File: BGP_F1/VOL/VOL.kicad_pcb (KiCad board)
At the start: 2 copper layers, 33 x 30 mm, 26 parts, among them P1 CONN_01X05, P2 CONN_01X05, P3 CONN_01X05, P4 CONN_01X03, P5 CONN_01X02, P7 CONN_01X12, U1 MC33178, U2 MC33178

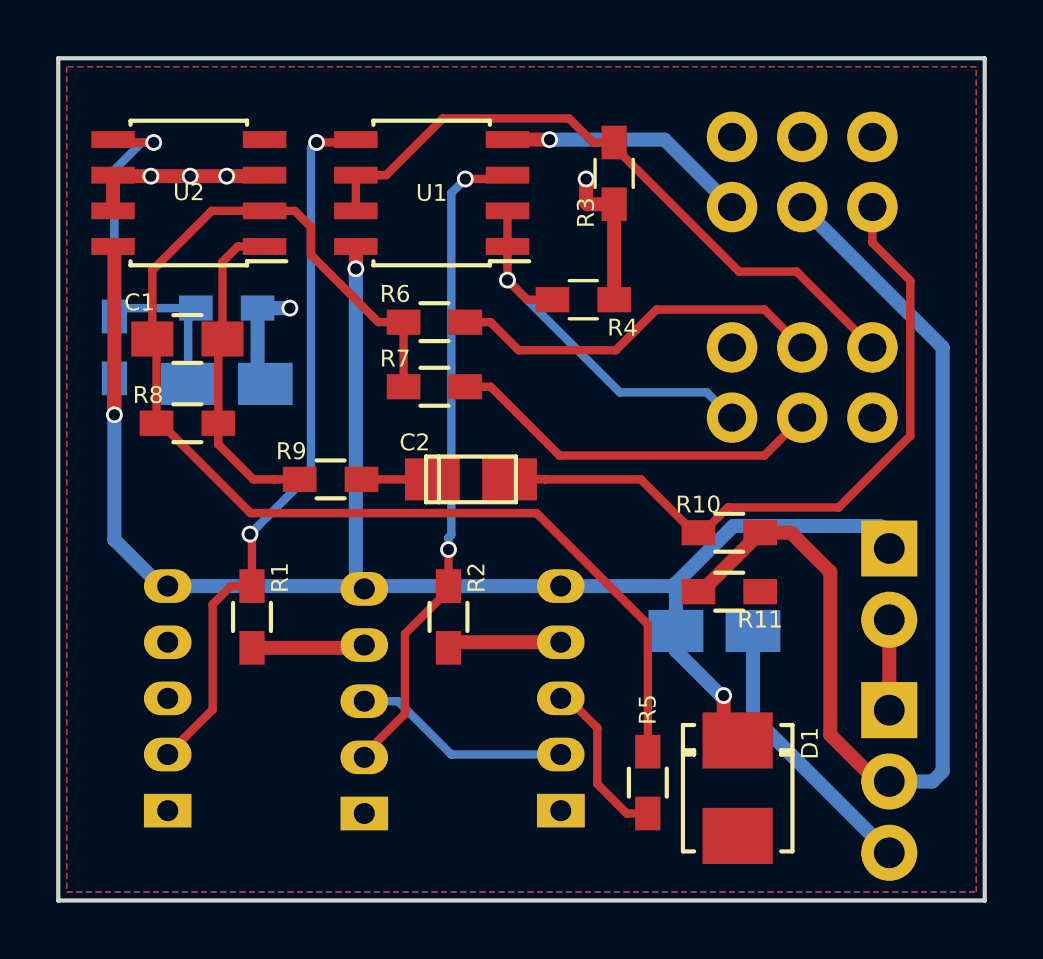
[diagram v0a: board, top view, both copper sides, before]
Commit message: HPF Done
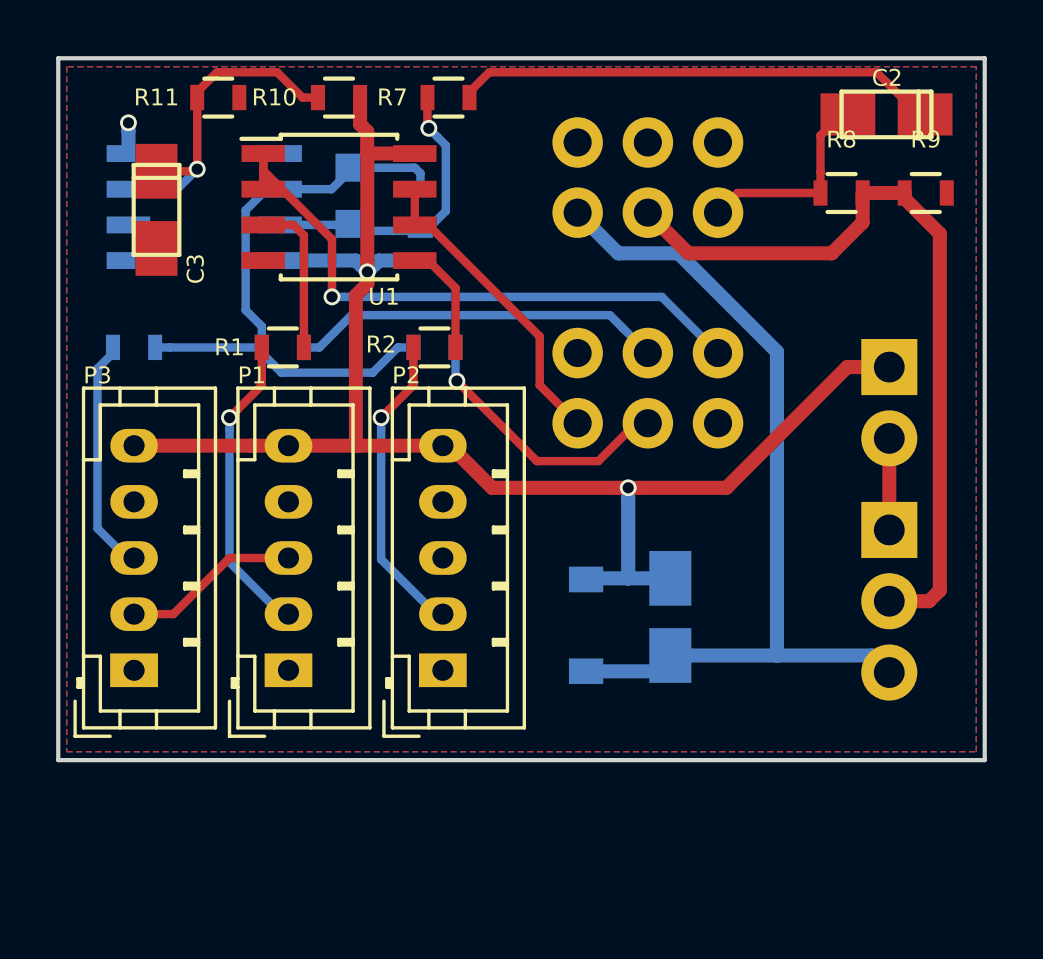
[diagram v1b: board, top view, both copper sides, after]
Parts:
- removed P7: CONN_01X12, LIBS:Potentiometer_Alps_RK097_Quad_Vertical_Dual_Shaft
- removed R12, R13: 100k, Resistors_SMD:R_0603_HandSoldering
- added P6: CONN_01X12, LIBS:Potentiometer_Alps_RK097_Quad_Vertical_Dual_Shaft, B.Cu at (155.5, 79.0)
- C1: footprint Capacitors_SMD:C_0805_HandSoldering -> Capacitors_SMD:C_0805; moved to B.Cu
- C3, P1, P2, P3: moved to F.Cu
- D1: footprint Diodes_SMD:DO-214BA -> Diodes_SMD:SOD-123; moved to B.Cu
- R1, R2: value 249k -> 100; footprint Resistors_SMD:R_0603_HandSoldering -> Resistors_SMD:R_0603
- R10: value 10k -> 100k; footprint Resistors_SMD:R_0603_HandSoldering -> Resistors_SMD:R_0603
- R11: value 12k -> 100k; footprint Resistors_SMD:R_0603_HandSoldering -> Resistors_SMD:R_0603
- R3, R4: value 11.1k -> 47k; footprint Resistors_SMD:R_0603_HandSoldering -> Resistors_SMD:R_0603; moved to B.Cu
- R5, R6: value 4.7k -> 47k; footprint Resistors_SMD:R_0603_HandSoldering -> Resistors_SMD:R_0603; moved to B.Cu
- R7: value 4.7k -> 100; footprint Resistors_SMD:R_0603_HandSoldering -> Resistors_SMD:R_0603
- R8: value 4.7k -> 10k; footprint Resistors_SMD:R_0603_HandSoldering -> Resistors_SMD:R_0603
- R9: value 100 -> 12k; footprint Resistors_SMD:R_0603_HandSoldering -> Resistors_SMD:R_0603
- U2: moved to B.Cu
- moved R11 25.3 mm to (142.7, 77.4)
- moved R8 24.7 mm to (164.9, 80.8), turned to 0 degrees
- moved R9 23.5 mm to (167.9, 80.8), turned to 0 degrees
- moved R10 20.8 mm to (147.0, 77.4), turned to 180 degrees
- moved C2 19.7 mm to (166.5, 78.0), turned to 0 degrees
- moved R3 18.2 mm to (139.7, 86.3), turned to 180 degrees
- moved R5 17.3 mm to (150.4, 86.3), turned to 0 degrees
- moved P3 16.0 mm to (139.7, 97.8)
- moved R4 10.8 mm to (145.0, 86.3), turned to 0 degrees
- moved R7 10.3 mm to (150.9, 77.4), turned to 180 degrees
- moved R1 9.66 mm to (145.0, 86.3), turned to 180 degrees
- moved R2 9.61 mm to (150.4, 86.3), turned to 180 degrees
- moved D1 7.92 mm to (155.8, 96.2)
- moved C1 7.80 mm to (147.5, 80.9), turned to 90 degrees
- moved C3 6.69 mm to (140.5, 81.4), turned to 90 degrees
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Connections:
- P3 pad 2: /BUF_B -> /BUF_N
- R1 pad 1: /OUT_N -> Net-(R1-Pad1)
- R1 pad 2: /Vref -> /OUT_N
- R10 pad 1: /PV_3 -> /V+
- R10 pad 2: /OUT -> Net-(C3-Pad1)
- R11 pad 1: /OUT -> Net-(C3-Pad1)
- R2 pad 1: /OUT_B -> Net-(R2-Pad1)
- R2 pad 2: /Vref -> /OUT_B
- R3 pad 1: /Vref -> Net-(C1-Pad2)
- R3 pad 2: /PB1_1 -> /OUT_HPF
- R4 pad 1: /Vref -> Net-(C1-Pad2)
- R4 pad 2: /PB2_1 -> /PB1_2
- R5 pad 2: /OUT_HPF -> /PB2_2
- R6 pad 1: Net-(C1-Pad2) -> Net-(C1-Pad1)
- R6 pad 2: /PB1_2 -> Net-(C1-Pad2)
- R7 pad 1: Net-(C1-Pad2) -> Net-(C2-Pad1)
- R7 pad 2: /PB2_2 -> Net-(C1-Pad1)
- R8 pad 1: Net-(C1-Pad1) -> /PV_3
- R8 pad 2: Net-(C1-Pad2) -> /OUT
- R9 pad 1: Net-(C2-Pad1) -> /OUT
- R9 pad 2: Net-(C1-Pad1) -> Earth
- U1 pad 1: /PB2_1 -> /PB1_1
- U1 pad 2: /PB2_1 -> /PB1_1
- U1 pad 3: /OUT_B -> Net-(R1-Pad1)
- U1 pad 5: /OUT_N -> Net-(R2-Pad1)
- U1 pad 6: /PB1_1 -> /PB2_1
- U1 pad 7: /PB1_1 -> /PB2_1
- U2 pad 1: Net-(C1-Pad1) -> /Vref
- U2 pad 2: Net-(C1-Pad2) -> /Vref
- U2 pad 3: /Vref -> Net-(C3-Pad1)
- U2 pad 5: Net-(C3-Pad1) -> /Vref
- U2 pad 6: /Vref -> Net-(C1-Pad2)
- U2 pad 7: /Vref -> Net-(C1-Pad1)
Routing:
- net Net-(C1-Pad2): track 44.9 -> 22.7 mm
- net /Vref: track 20.1 -> 0.00 mm, vias 4 -> 0
- net /PV_3: track 25.2 -> 7.28 mm
- net /OUT_N: track 25.9 -> 11.0 mm, vias 2 -> 1
- net Net-(C2-Pad1): track 2.53 -> 17.3 mm
- net /OUT_B: track 23.5 -> 11.0 mm, vias 2 -> 1
- net /OUT: track 39.0 -> 27.9 mm
- net Earth: track 23.7 -> 32.4 mm, vias 2 -> 1
- net /BUF_B: track 7.99 -> 0.00 mm
- net /BUF_N: track 0.00 -> 6.33 mm
- net Net-(R1-Pad1): track 0.00 -> 5.60 mm
- net /V+: track 59.8 -> 55.1 mm, vias 3 -> 2
- net Net-(R2-Pad1): track 0.00 -> 3.97 mm
- net /PB2_2: track 13.6 -> 10.1 mm, vias 0 -> 1
- net /PB2_1: track 14.4 -> 11.0 mm, vias 1 -> 0
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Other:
- board size 33 x 30 mm -> 33 x 25 mm
